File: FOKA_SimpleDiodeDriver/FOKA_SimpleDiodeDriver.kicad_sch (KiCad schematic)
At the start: 22 parts, among them J1 IN, J2 Conn_01x02, Q2 BJT, U2 ADA4891-1

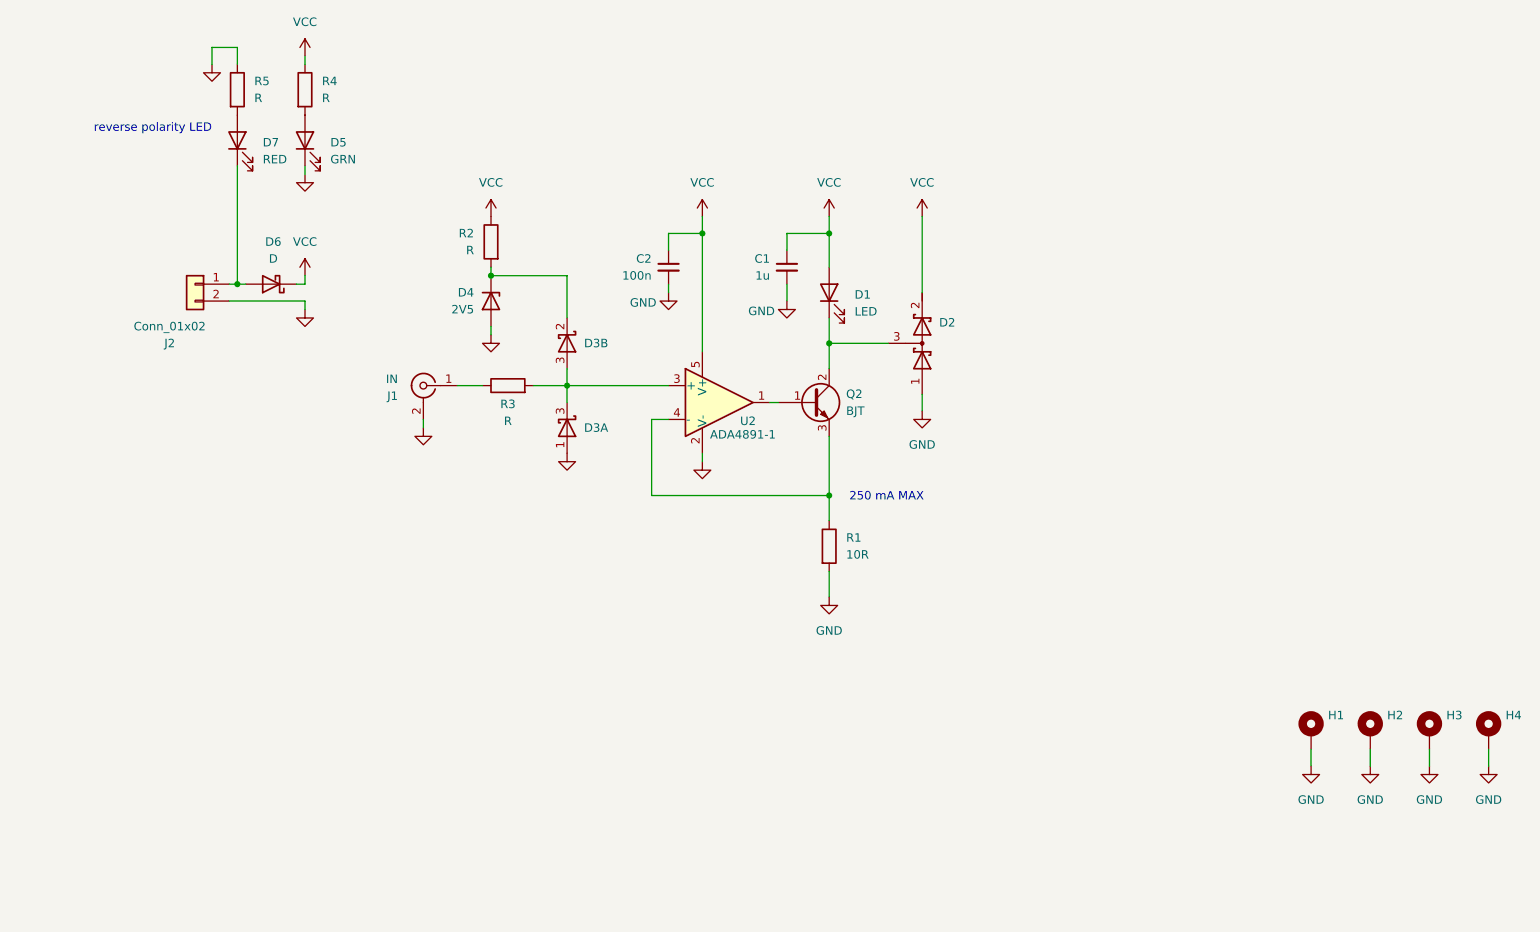
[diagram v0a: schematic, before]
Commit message: v0.9
awaiting pre-production review
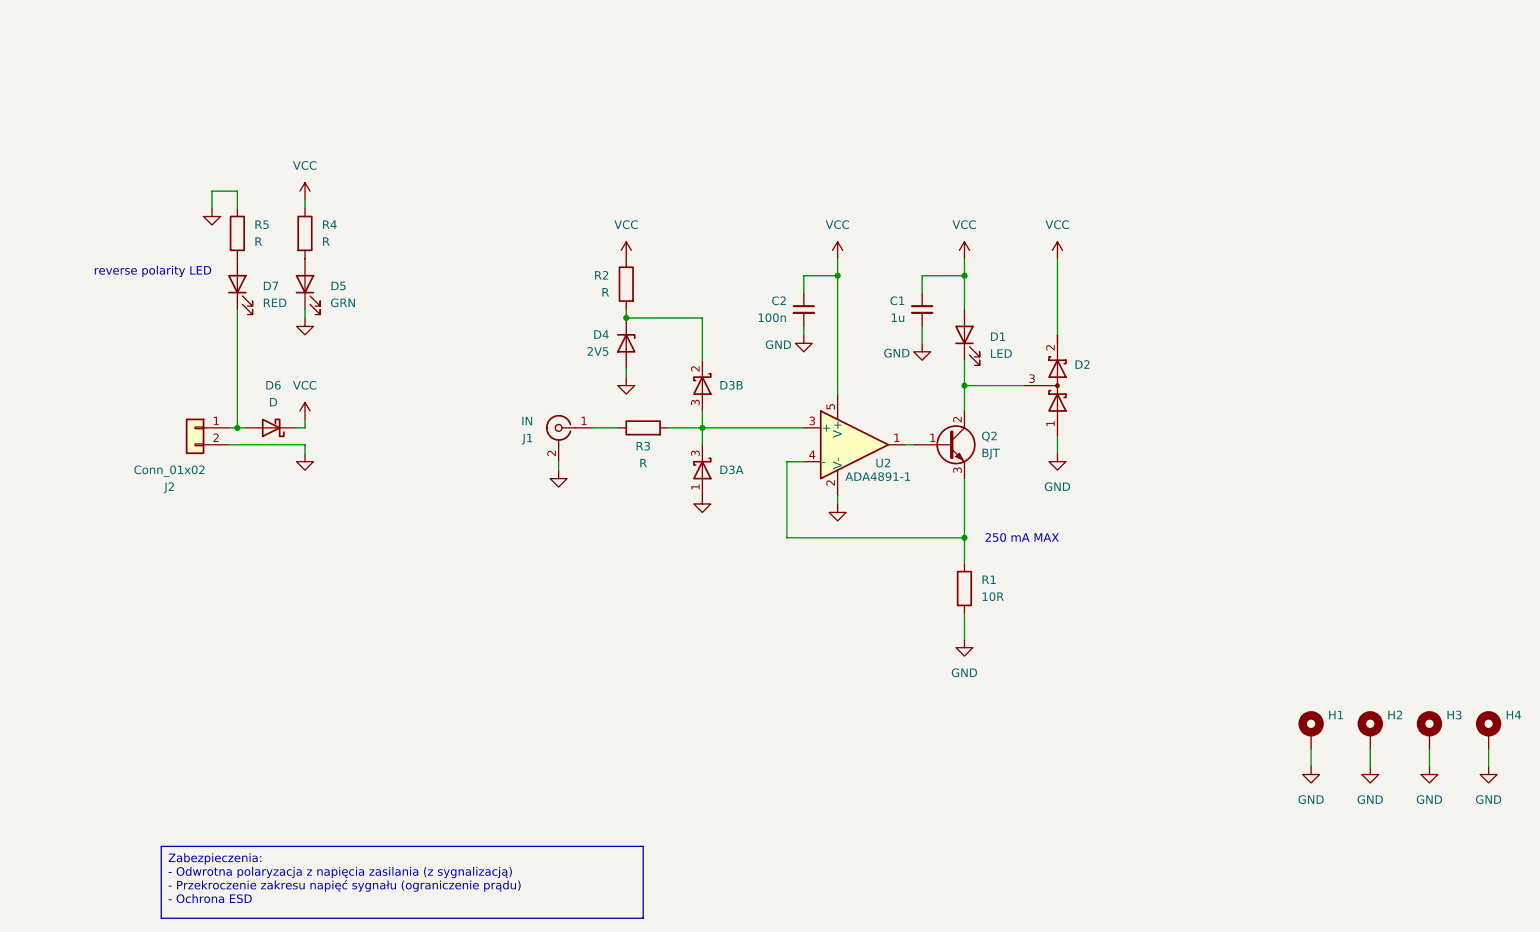
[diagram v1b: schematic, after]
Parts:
- J2: footprint Power_Connectors:691311500102 -> Power_Connectors:691313510002
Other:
- company: (none) -> KN FOKA
- title: (none) -> Zabezpieczony sterownik diody IR
- moved on the sheet: C1, C2, D1, D2, D3A, D3B, D4, D5, D6, D7, J1, J2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

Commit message: minor updates
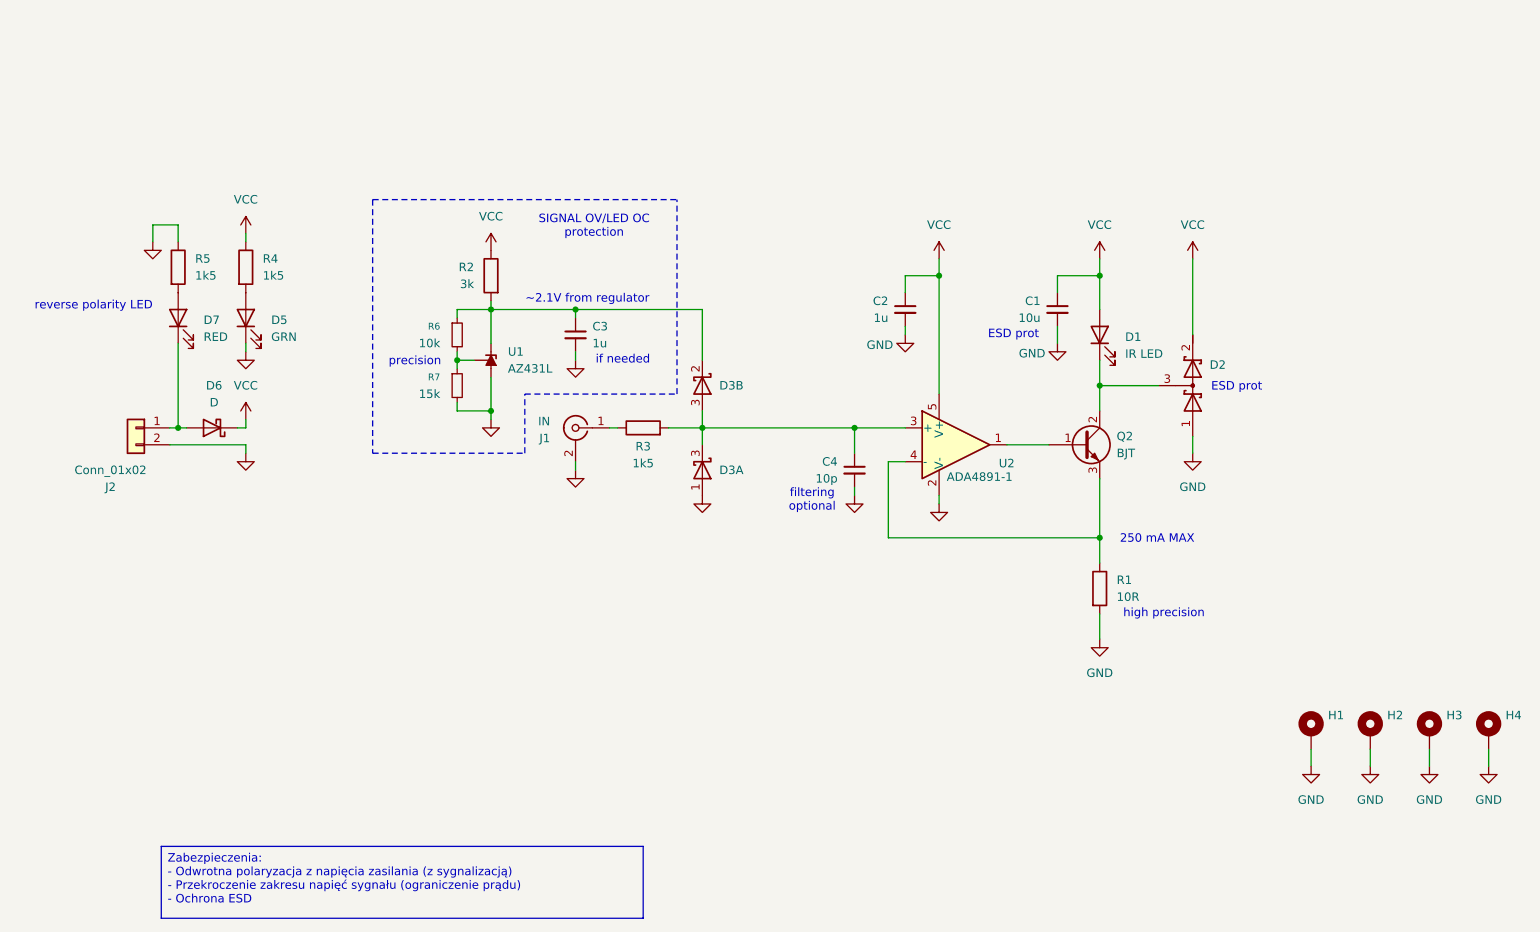
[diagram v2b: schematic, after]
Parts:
- removed D4: 2V5, Diode_SMD:D_SOD-323_HandSoldering, symbol Device:D_Zener
- added C3: 1u, Capacitor_SMD:C_0603_1608Metric_Pad1.08x0.95mm_HandSolder, symbol Device:C_Small
- added C4: 10p, Capacitor_SMD:C_0603_1608Metric_Pad1.08x0.95mm_HandSolder, symbol Device:C_Small
- added R6: 10k, symbol Device:R_Small
- added R7: 15k, symbol Device:R_Small
- added U1: AZ431L, Package_TO_SOT_SMD:SOT-23, symbol Reference_Voltage:TL432DBZ
- C1: value 1u -> 10u
- C2: value 100n -> 1u
- D1: value LED -> IR LED
- R2: value R -> 3k
- R3, R4, R5: value R -> 1k5
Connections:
- net GND: now also C3.2, C4.2, R7.2, U1.3 (A)
- net at D3.2 (K), R2.2: now also C3.1, R6.1, U1.2 (K)
- net at D3.3 (K), D3.3 (K), R3.2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: now also C4.1
- new net: R6.2, R7.1, U1.1 (REF)
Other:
- note added: "ESD prot"
- note added: "SIGNAL OV/LED OC protection"
- note added: "filtering optional"
- note added: "high precision"
- note added: "if needed"
- note added: "precision"
- note added: "~2.1V from regulator"
- moved on the sheet: C1, C2, D1, D2, D5, D6, D7, J1, J2, Q2, R1, R2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
